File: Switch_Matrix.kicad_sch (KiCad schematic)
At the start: 54 parts, among them SW10 MX Hotswap, SW11 MX Hotswap, SW12 MX Hotswap, SW13 MX Hotswap, SW14 MX Hotswap, SW15 MX Hotswap, SW16 MX Hotswap, SW17 MX Hotswap, SW18 MX Hotswap, SW19 MX Hotswap, SW2 MX Hotswap, SW20 MX Hotswap, SW21 MX Hotswap, SW22 MX Hotswap, SW23 MX Hotswap, SW24 MX Hotswap, SW25 MX Hotswap, SW26 MX Hotswap, SW27 MX Hotswap, SW28 MX Hotswap, SW3 MX Hotswap, SW4 MX Hotswap, SW5 MX Hotswap, SW6 MX Hotswap, SW7 MX Hotswap, SW8 MX Hotswap, SW9 MX Hotswap

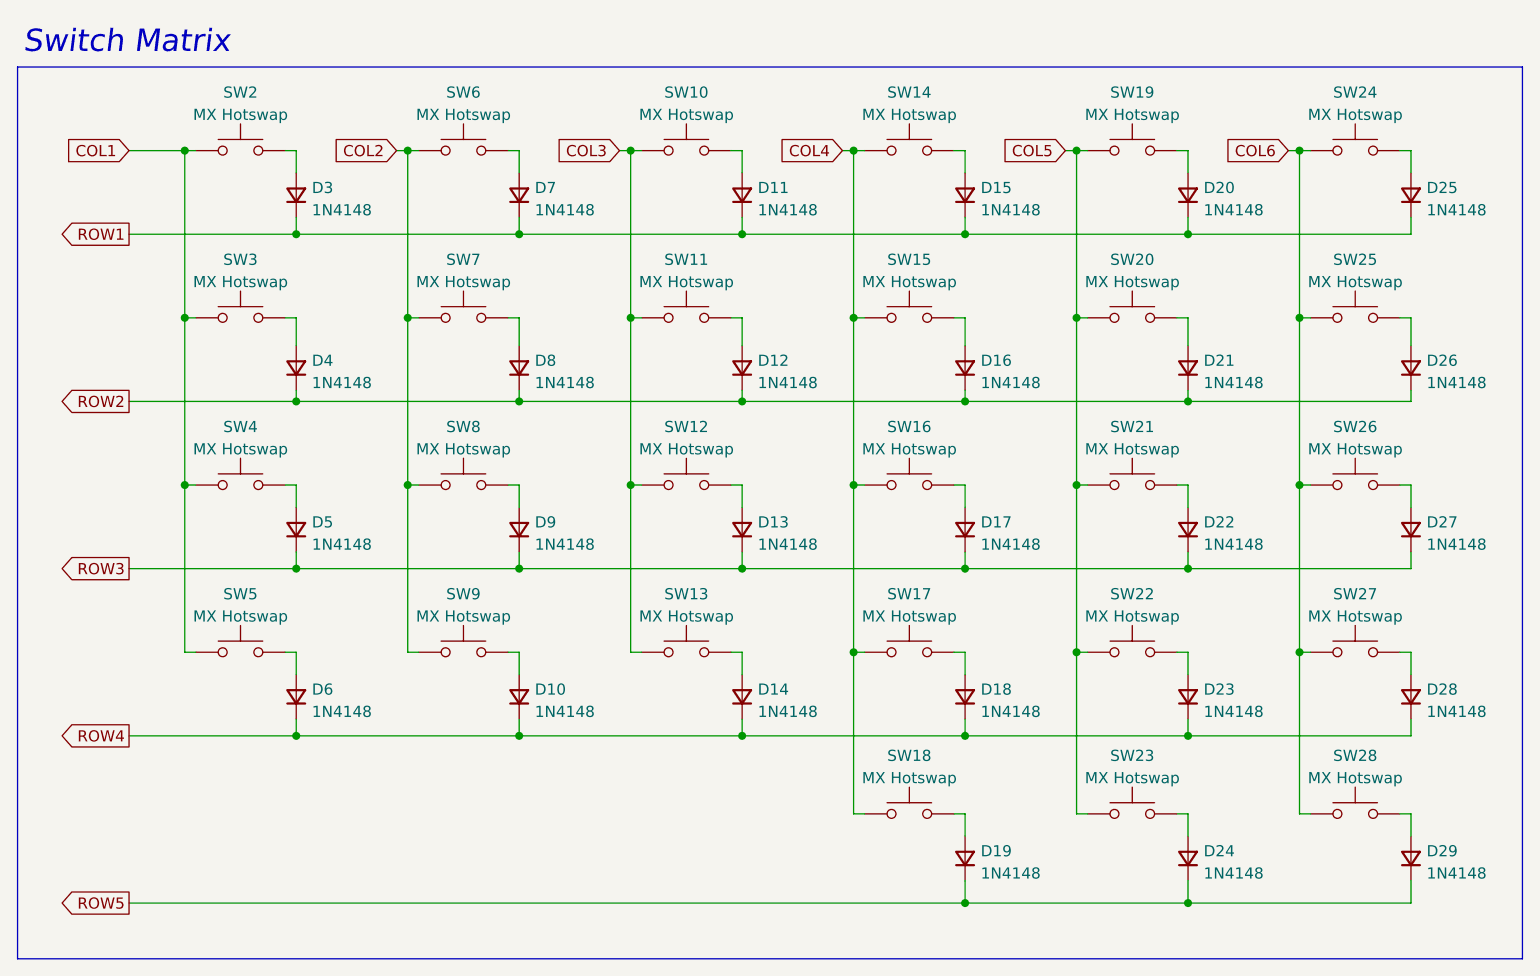
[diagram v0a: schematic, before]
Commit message: feat(pcb): Switch from 4.3mm NPTH mounting holes to M2 PTH
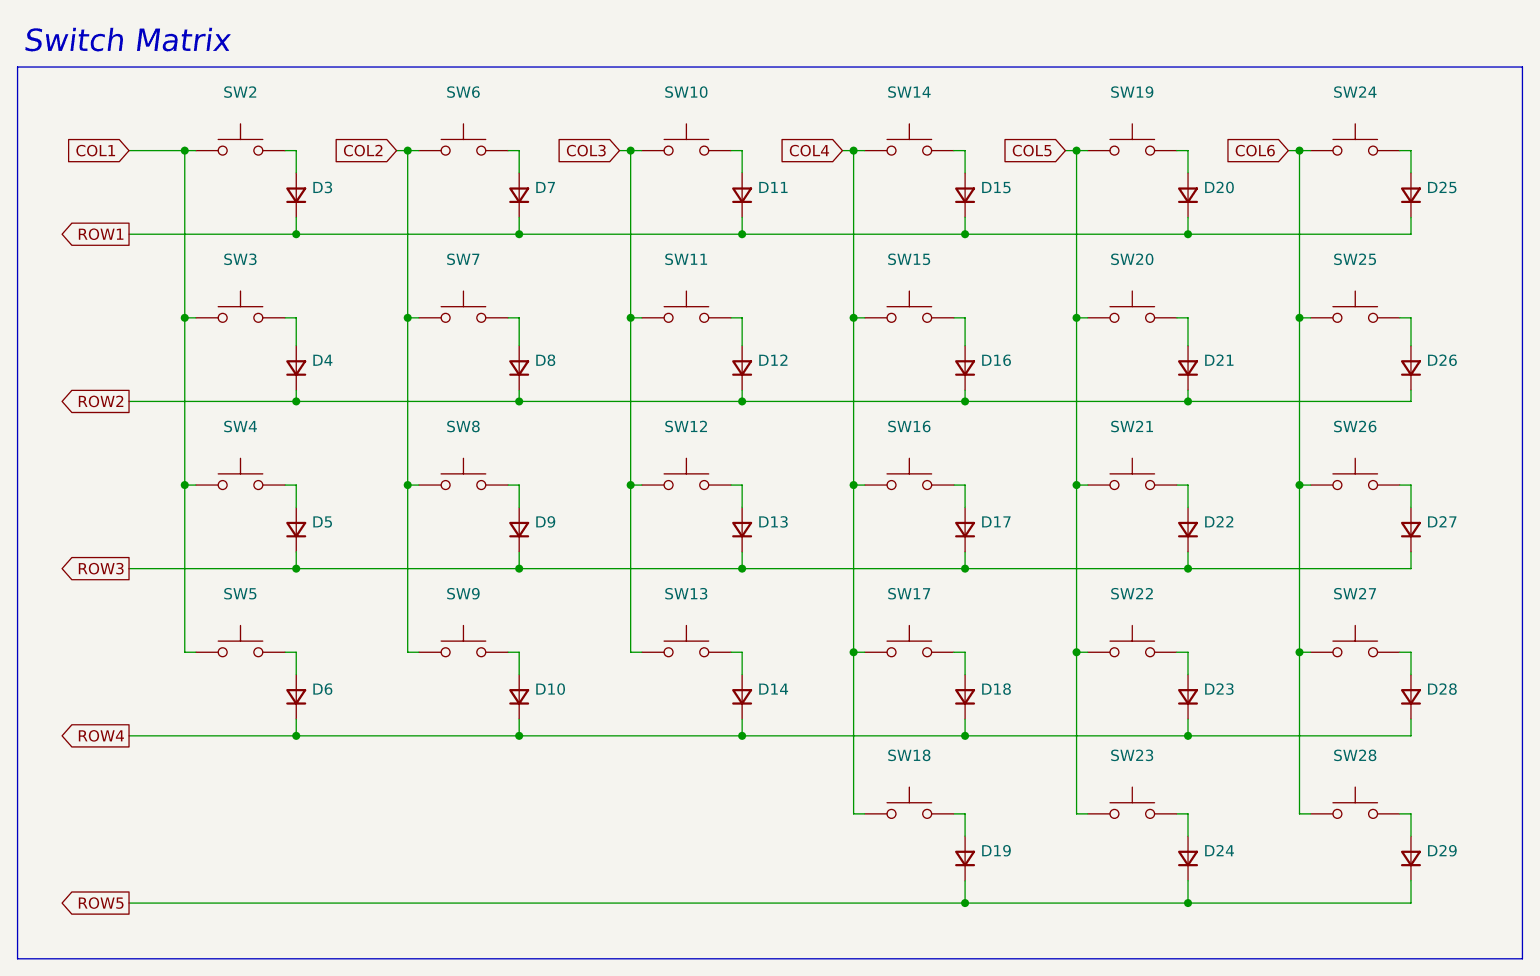
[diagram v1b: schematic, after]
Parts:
- D10, D11, D12, D13, D14, D15, D16, D17, D18, D19, D20, D21, D22, D23, D24, D25, D26, D27, D28, D29, D3, D4, D5, D6, D7, D8, D9: value 1N4148 -> (none); footprint Conejo:D_SOD-523 (Reversible) -> (none)
- SW10, SW11, SW12, SW13, SW14, SW15, SW16, SW17, SW18, SW19, SW2, SW20, SW21, SW22, SW23, SW24, SW25, SW26, SW27, SW3, SW4, SW5, SW6, SW7, SW8, SW9: value MX Hotswap -> (none); footprint Conejo:MXOnly-1U-Hotswap (Reversible) -> (none)
- SW28: value MX Hotswap -> (none); footprint Conejo:MXOnly-1.5U-Hotswap (Reversible) -> (none)

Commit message: feat(pcb): Version 1.0.0
- Change decoupling capacitors from 4.7uF/1uF pairs to both 4.7uF
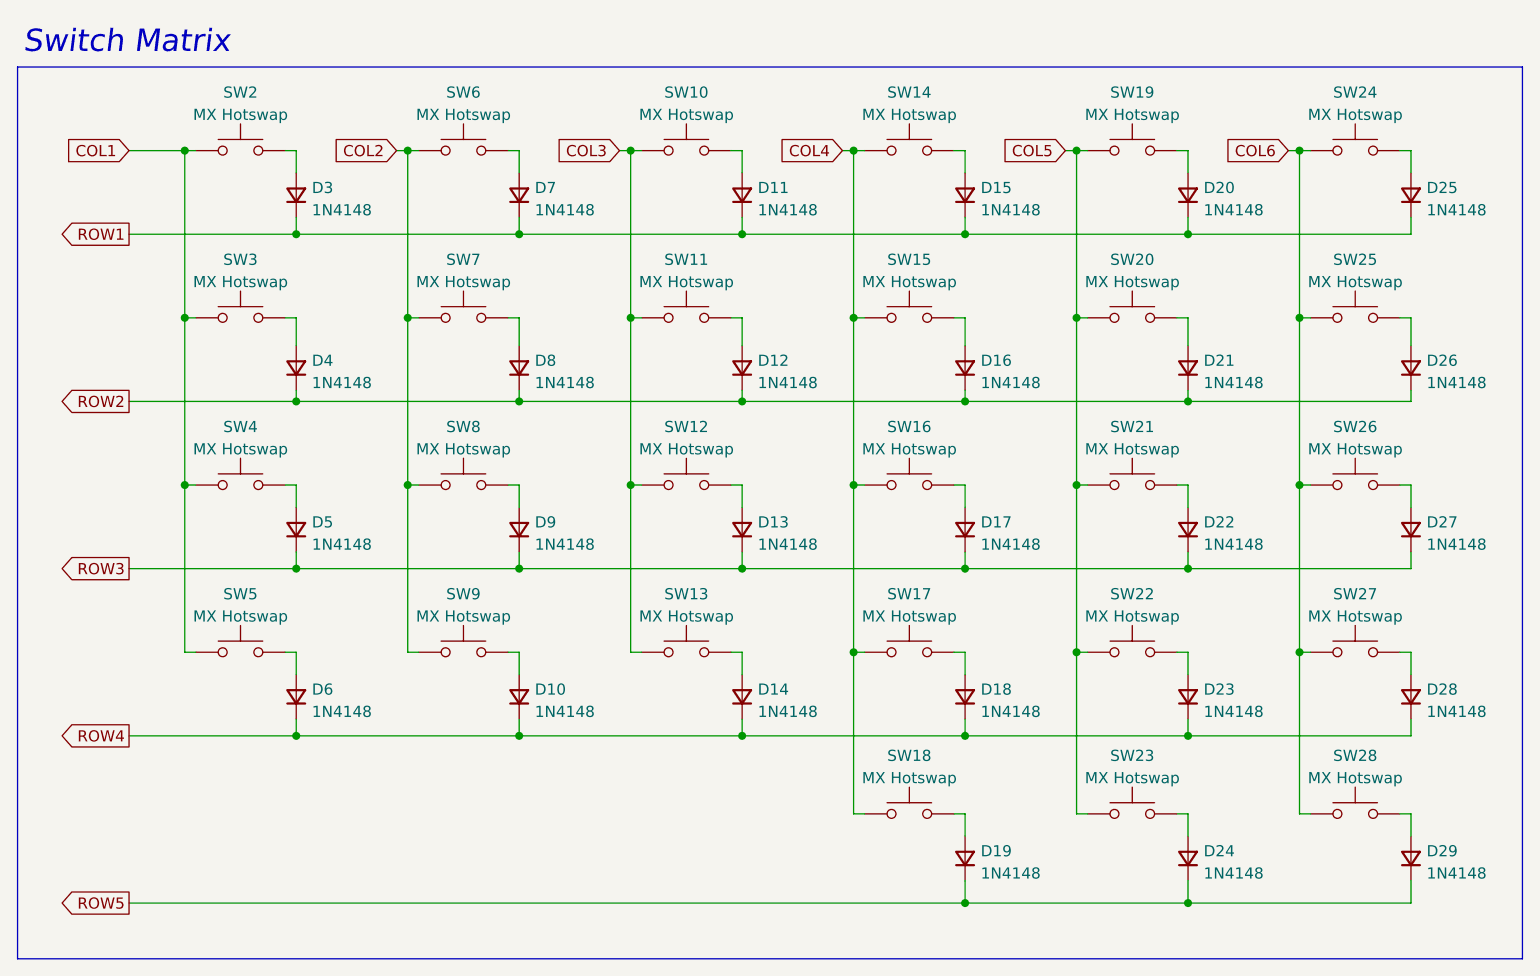
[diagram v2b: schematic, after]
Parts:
- D10, D11, D12, D13, D14, D15, D16, D17, D18, D19, D20, D21, D22, D23, D24, D25, D26, D27, D28, D29, D3, D4, D5, D6, D7, D8, D9: value (none) -> 1N4148; footprint (none) -> Conejo:D_SOD-523 (Reversible)
- SW10, SW11, SW12, SW13, SW14, SW15, SW16, SW17, SW18, SW19, SW2, SW20, SW21, SW22, SW23, SW24, SW25, SW26, SW27, SW3, SW4, SW5, SW6, SW7, SW8, SW9: value (none) -> MX Hotswap; footprint (none) -> Conejo:MXOnly-1U-Hotswap (Reversible)
- SW28: value (none) -> MX Hotswap; footprint (none) -> Conejo:MXOnly-1.5U-Hotswap (Reversible)
